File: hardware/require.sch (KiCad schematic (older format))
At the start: 0 parts

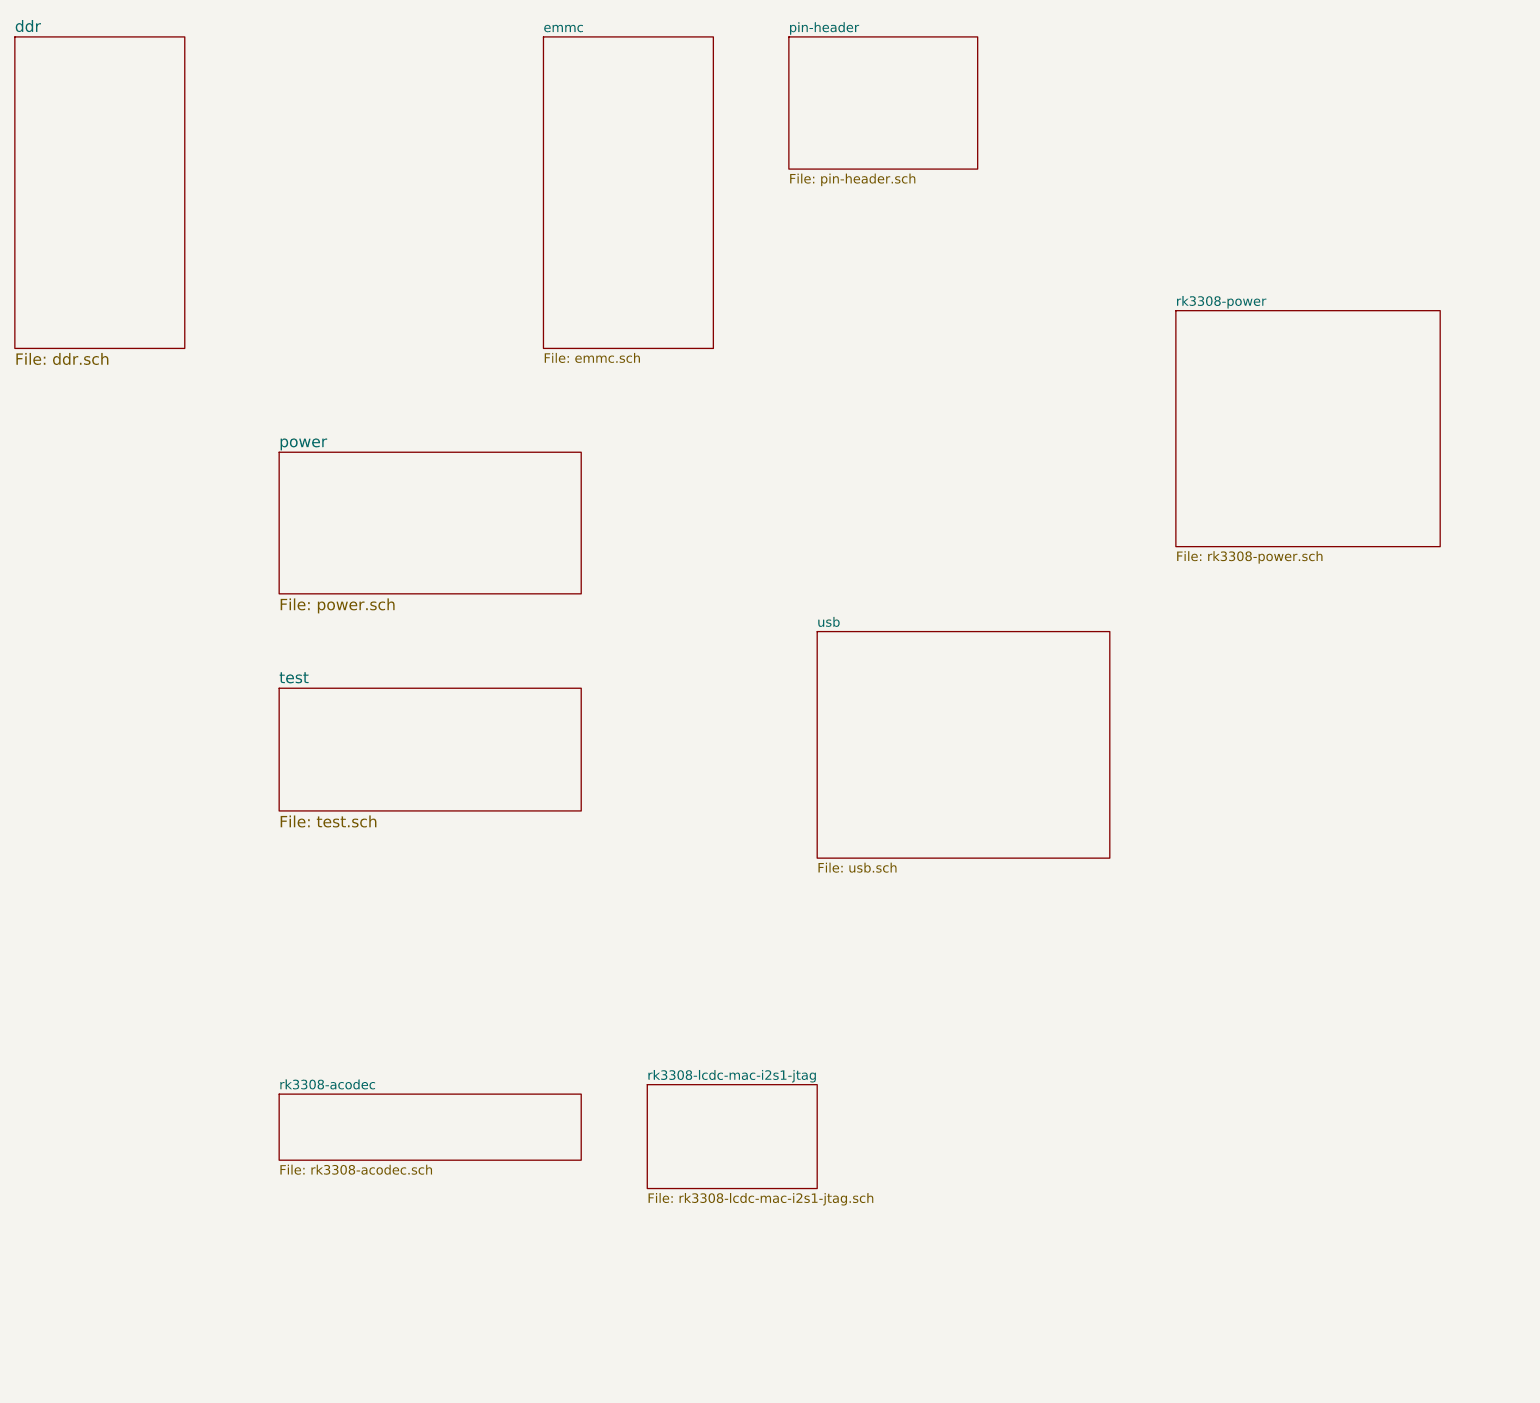
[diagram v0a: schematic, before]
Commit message: wip
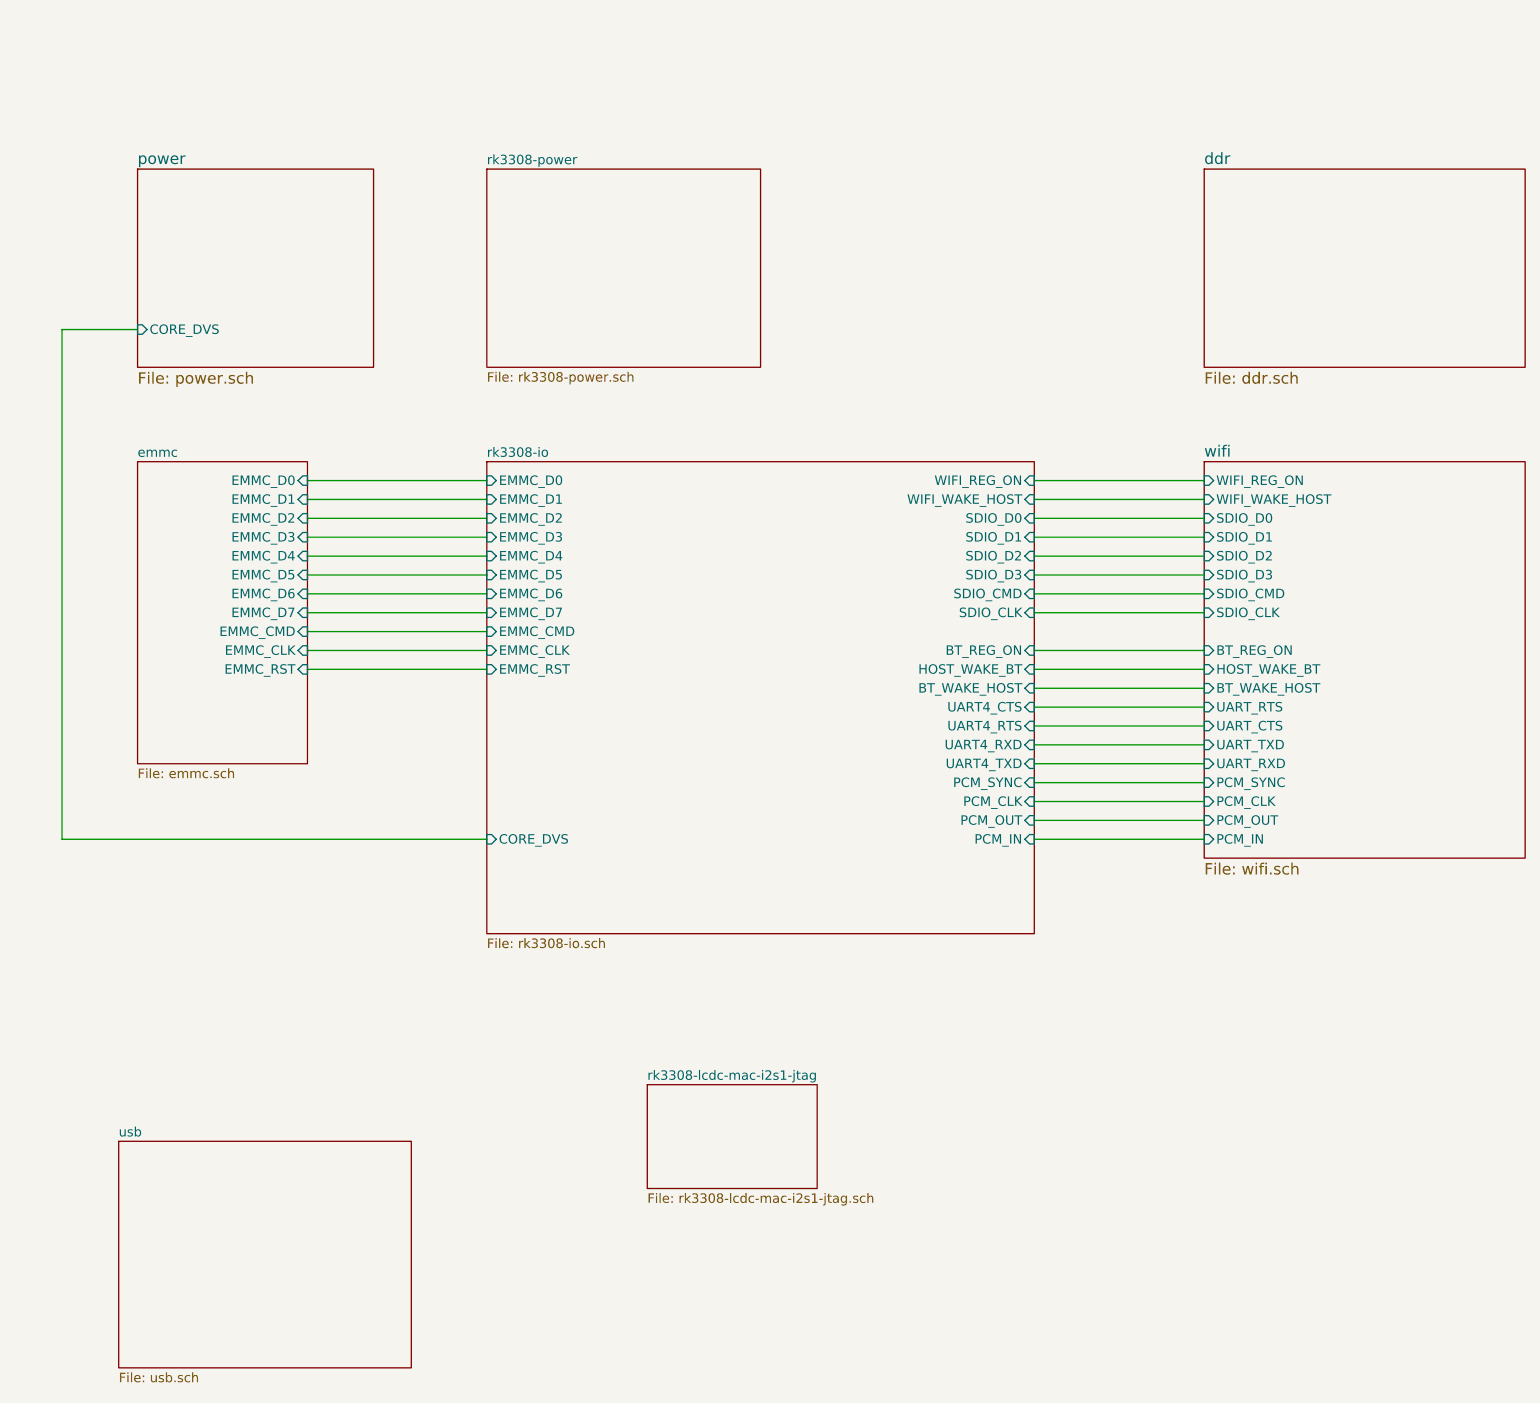
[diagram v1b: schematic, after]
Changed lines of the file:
@@
 EELAYER 26 0
 EELAYER END
-$Descr A4 11693 8268
+$Descr A3 16535 11693
 encoding utf-8
-Sheet 1 10
+Sheet 1 9
 Title ""
 Date ""
@@
 $EndDescr
 $Sheet
-S 2650 3150 1600 750
+S 1900 1650 1250 1050
 U 5C2CD8AE
 F0 "power" 60
 F1 "power.sch" 60
+F2 "CORE_DVS" I L 1900 2500 50
 $EndSheet
 $Sheet
-S 2650 4400 1600 650
+S 7550 3200 1700 2100
 U 5C2D00B3
-F0 "test" 60
-F1 "test.sch" 60
+F0 "wifi" 60
+F1 "wifi.sch" 60
+F2 "HOST_WAKE_BT" I L 7550 4300 50
+F3 "BT_WAKE_HOST" I L 7550 4400 50
+F4 "WIFI_REG_ON" I L 7550 3300 50
+F5 "WIFI_WAKE_HOST" I L 7550 3400 50
+F6 "SDIO_D0" I L 7550 3500 50
+F7 "SDIO_D1" I L 7550 3600 50
+F8 "SDIO_D2" I L 7550 3700 50
+F9 "SDIO_D3" I L 7550 3800 50
+F10 "SDIO_CMD" I L 7550 3900 50
+F11 "SDIO_CLK" I L 7550 4000 50
+F12 "BT_REG_ON" I L 7550 4200 50
+F13 "UART_RTS" I L 7550 4500 50
+F14 "UART_CTS" I L 7550 4600 50
+F15 "UART_TXD" I L 7550 4700 50
+F16 "UART_RXD" I L 7550 4800 50
+F17 "PCM_SYNC" I L 7550 4900 50
+F18 "PCM_CLK" I L 7550 5000 50
+F19 "PCM_OUT" I L 7550 5100 50
+F20 "PCM_IN" I L 7550 5200 50
 $EndSheet
 $Sheet
-S 1250 950  900  1650
+S 7550 1650 1700 1050
 U 5C2F0873
 F0 "ddr" 60
@@
 $EndSheet
 $Sheet
-S 7400 2400 1400 1250
+S 3750 1650 1450 1050
 U 5C325762
 F0 "rk3308-power" 50
@@
 $EndSheet
 $Sheet
-S 2650 6550 1600 350
-U 5C46A4DA
-F0 "rk3308-acodec" 50
-F1 "rk3308-acodec.sch" 50
-$EndSheet
-$Sheet
-S 4050 950  900  1650
+S 1900 3200 900  1600
 U 5CDAE2B6
 F0 "emmc" 50
 F1 "emmc.sch" 50
+F2 "EMMC_RST" I R 2800 4300 50
+F3 "EMMC_D0" I R 2800 3300 50
+F4 "EMMC_D1" I R 2800 3400 50
+F5 "EMMC_D2" I R 2800 3500 50
+F6 "EMMC_D3" I R 2800 3600 50
+F7 "EMMC_D4" I R 2800 3700 50
+F8 "EMMC_D5" I R 2800 3800 50
+F9 "EMMC_D6" I R 2800 3900 50
+F10 "EMMC_D7" I R 2800 4000 50
+F11 "EMMC_CMD" I R 2800 4100 50
+F12 "EMMC_CLK" I R 2800 4200 50
 $EndSheet
 $Sheet
@@
 $EndSheet
 $Sheet
-S 5500 4100 1550 1200
+S 1800 6800 1550 1200
 U 5CED3BD3
 F0 "usb" 50
@@
 $EndSheet
 $Sheet
-S 5350 950  1000 700
-U 5C48B775
-F0 "pin-header" 50
-F1 "pin-header.sch" 50
+S 3750 3200 2900 2500
+U 5C87E279
+F0 "rk3308-io" 50
+F1 "rk3308-io.sch" 50
+F2 "EMMC_RST" I L 3750 4300 50
+F3 "EMMC_D0" I L 3750 3300 50
+F4 "EMMC_D1" I L 3750 3400 50
+F5 "EMMC_D2" I L 3750 3500 50
+F6 "EMMC_D3" I L 3750 3600 50
+F7 "EMMC_D4" I L 3750 3700 50
+F8 "EMMC_D5" I L 3750 3800 50
+F9 "EMMC_D6" I L 3750 3900 50
+F10 "EMMC_D7" I L 3750 4000 50
+F11 "EMMC_CMD" I L 3750 4100 50
+F12 "EMMC_CLK" I L 3750 4200 50
+F13 "WIFI_REG_ON" I R 6650 3300 50
+F14 "WIFI_WAKE_HOST" I R 6650 3400 50
+F15 "SDIO_D0" I R 6650 3500 50
+F16 "SDIO_D1" I R 6650 3600 50
+F17 "SDIO_D2" I R 6650 3700 50
+F18 "SDIO_D3" I R 6650 3800 50
+F19 "SDIO_CMD" I R 6650 3900 50
+F20 "SDIO_CLK" I R 6650 4000 50
+F21 "BT_REG_ON" I R 6650 4200 50
+F22 "HOST_WAKE_BT" I R 6650 4300 50
+F23 "BT_WAKE_HOST" I R 6650 4400 50
+F24 "UART4_CTS" I R 6650 4500 50
+F25 "UART4_RTS" I R 6650 4600 50
+F26 "UART4_RXD" I R 6650 4700 50
+F27 "UART4_TXD" I R 6650 4800 50
+F28 "PCM_SYNC" I R 6650 4900 50
+F29 "PCM_CLK" I R 6650 5000 50
+F30 "PCM_OUT" I R 6650 5100 50
+F31 "PCM_IN" I R 6650 5200 50
+F32 "CORE_DVS" I L 3750 5200 50
 $EndSheet
+Wire Wire Line
+	2800 3300 3750 3300
+Wire Wire Line
+	2800 3400 3750 3400
+Wire Wire Line
+	2800 3500 3750 3500
+Wire Wire Line
+	2800 3600 3750 3600
+Wire Wire Line
+	2800 3700 3750 3700
+Wire Wire Line
+	2800 3800 3750 3800
+Wire Wire Line
+	2800 3900 3750 3900
+Wire Wire Line
+	2800 4000 3750 4000
+Wire Wire Line
+	2800 4100 3750 4100
+Wire Wire Line
+	2800 4200 3750 4200
+Wire Wire Line
+	2800 4300 3750 4300
+Wire Wire Line
+	6650 3300 7550 3300
+Wire Wire Line
+	6650 3400 7550 3400
+Wire Wire Line
+	6650 3500 7550 3500
+Wire Wire Line
+	6650 3600 7550 3600
+Wire Wire Line
+	6650 3700 7550 3700
+Wire Wire Line
+	6650 3800 7550 3800
+Wire Wire Line
+	6650 3900 7550 3900
+Wire Wire Line
+	6650 4000 7550 4000
+Wire Wire Line
+	7550 4200 6650 4200
+Wire Wire Line
+	7550 4300 6650 4300
+Wire Wire Line
+	6650 4400 7550 4400
+Wire Wire Line
+	6650 4500 7550 4500
+Wire Wire Line
+	6650 4600 7550 4600
+Wire Wire Line
+	6650 4700 7550 4700
+Wire Wire Line
+	6650 4800 7550 4800
+Wire Wire Line
+	6650 4900 7550 4900
+Wire Wire Line
+	6650 5000 7550 5000
+Wire Wire Line
+	6650 5100 7550 5100
+Wire Wire Line
+	6650 5200 7550 5200
+Wire Wire Line
+	1900 2500 1500 2500
+Wire Wire Line
+	1500 2500 1500 5200
+Wire Wire Line
+	1500 5200 3750 5200
 $EndSCHEMATC
